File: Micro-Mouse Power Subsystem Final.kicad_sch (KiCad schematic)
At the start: 67 parts, among them J3 USB_C_Receptacle_USB2.0_16P, J4 Battery terminals, J5 Conn_02x16_Odd_Even, Q1 DMP3099L, Q2 2N7002, Q3 DMP3099L, SW1 SW_SPDT, U1 DRV8833PWP, U13 INA219AxD, U2 DRV8833PWP, U3 CH224K, U4 AMS1117-3.3, U5 MT3608, U6 TP4056-42-ESOP8, U7 AMS1117-5.0

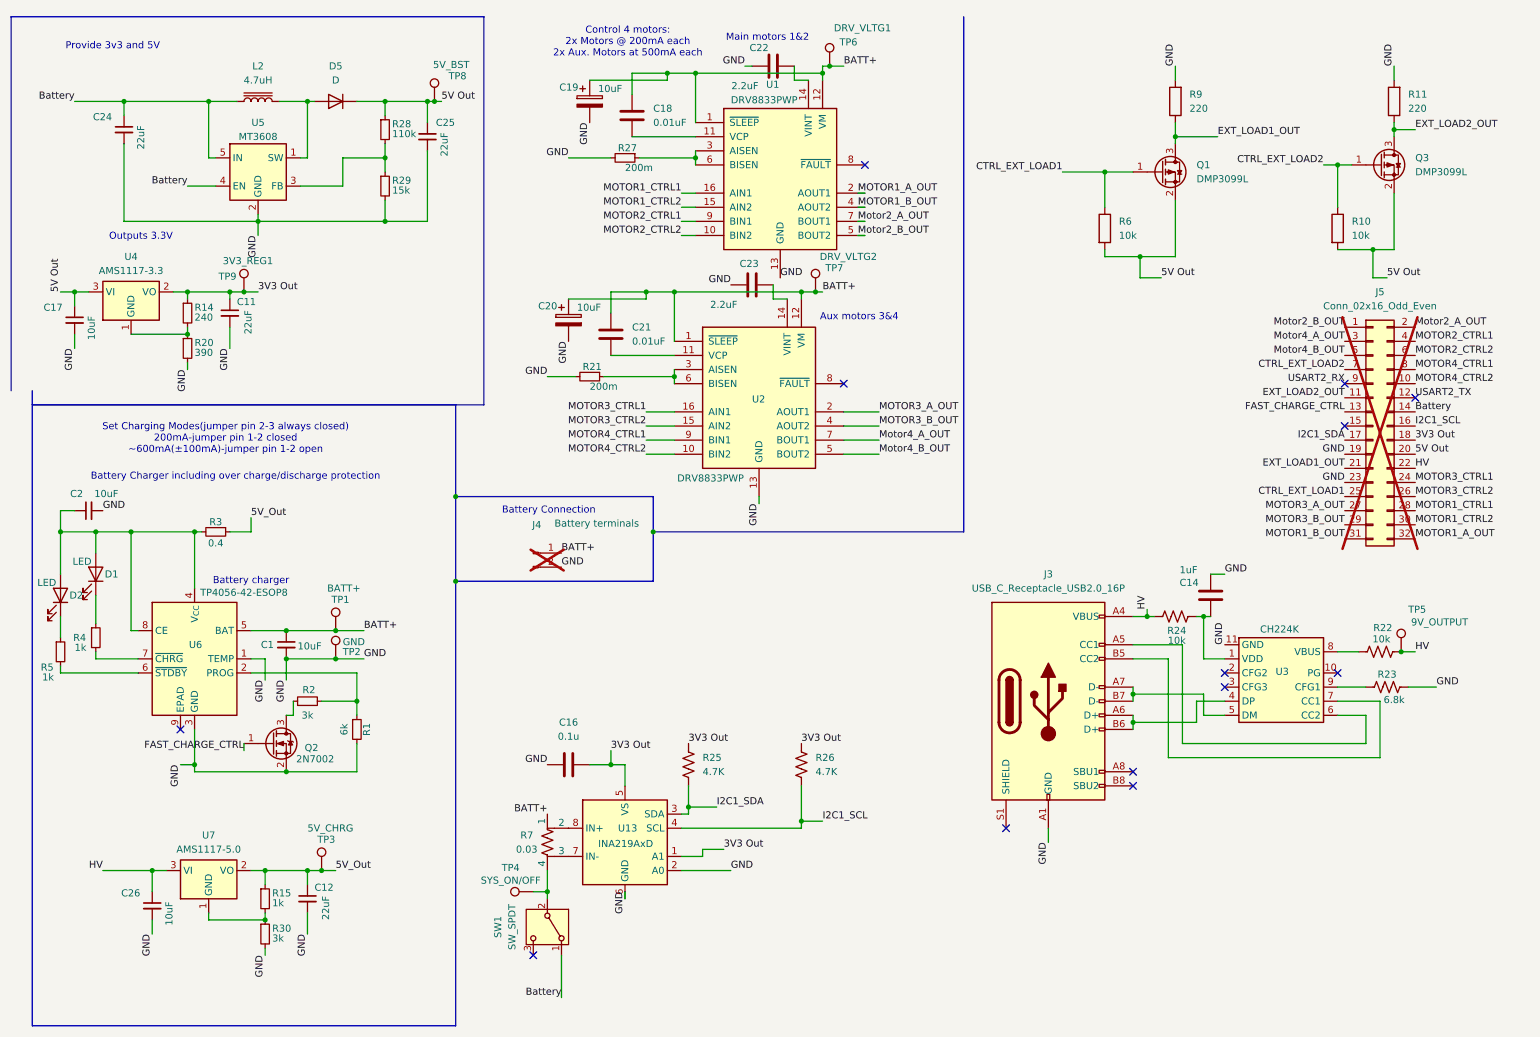
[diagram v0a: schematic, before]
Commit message: Add files via upload
updating the schematic
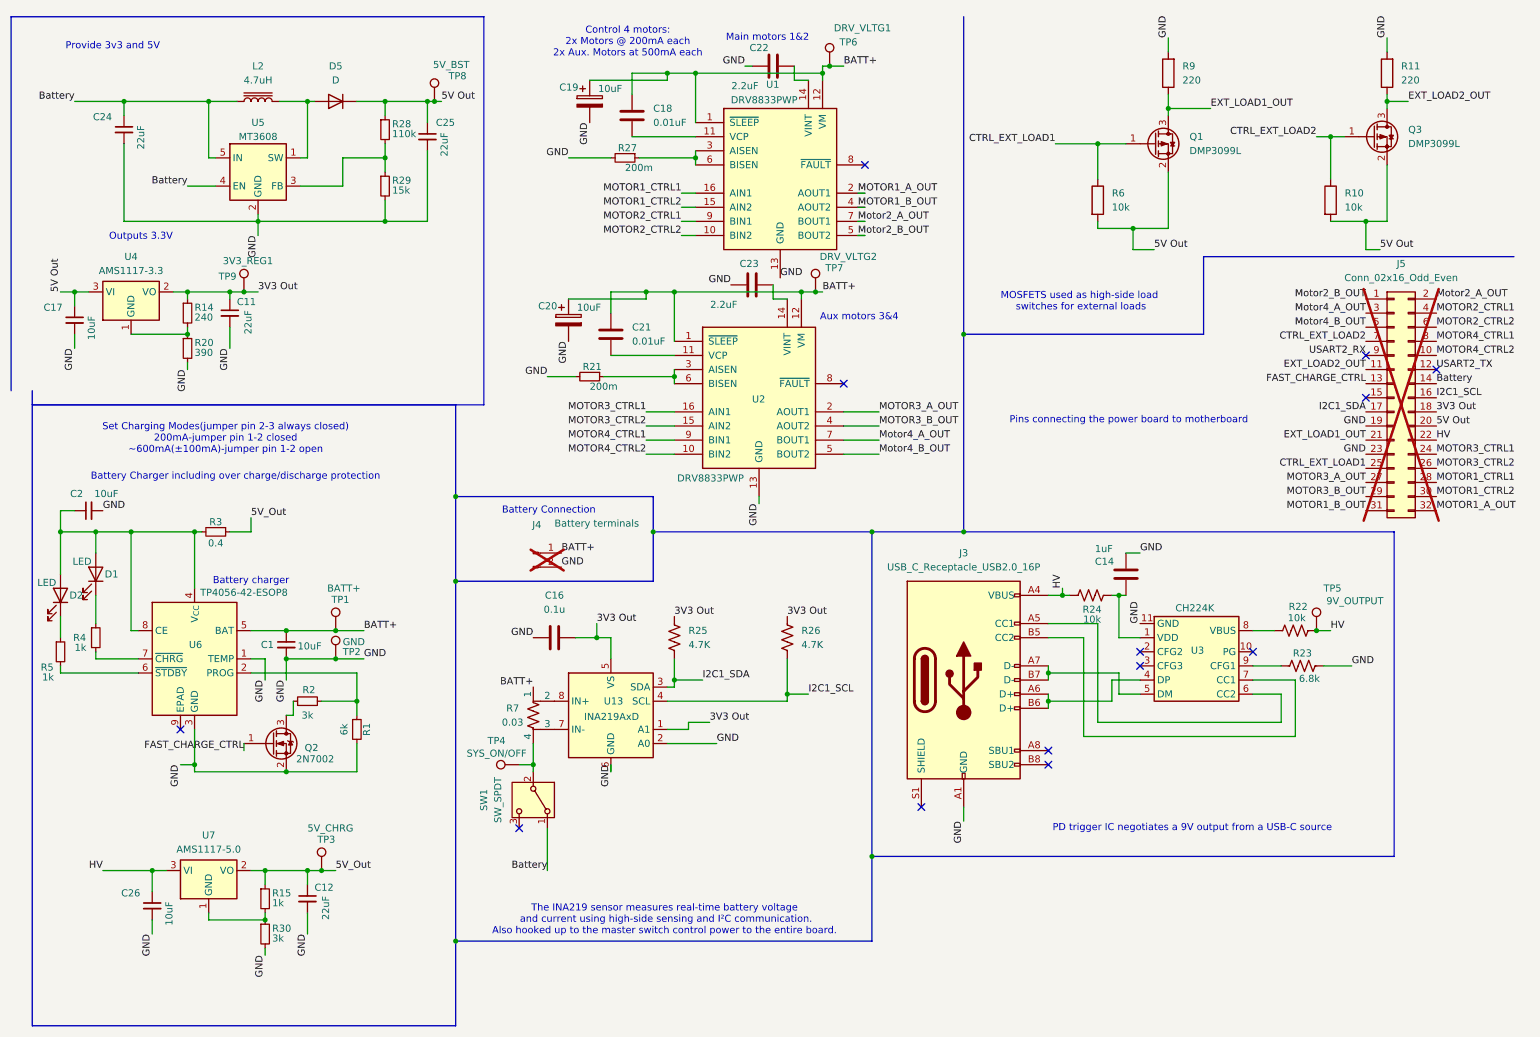
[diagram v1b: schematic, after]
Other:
- note added: "MOSFETS used as high-side load switches for external loads"
- note added: "PD trigger IC negotiates a 9V output from a USB-C source"
- note added: "Pins connecting the power board to motherboard"
- note added: "The INA219 sensor measures real-time battery voltage and current using high-side sensing and I²C communication. Also hooked up to the master switch control power to the entire board."
- moved on the sheet: C14, C16, J3, J5, Q1, Q3, R10, R11, R22, R23, R24, R25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

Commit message: Add files via upload
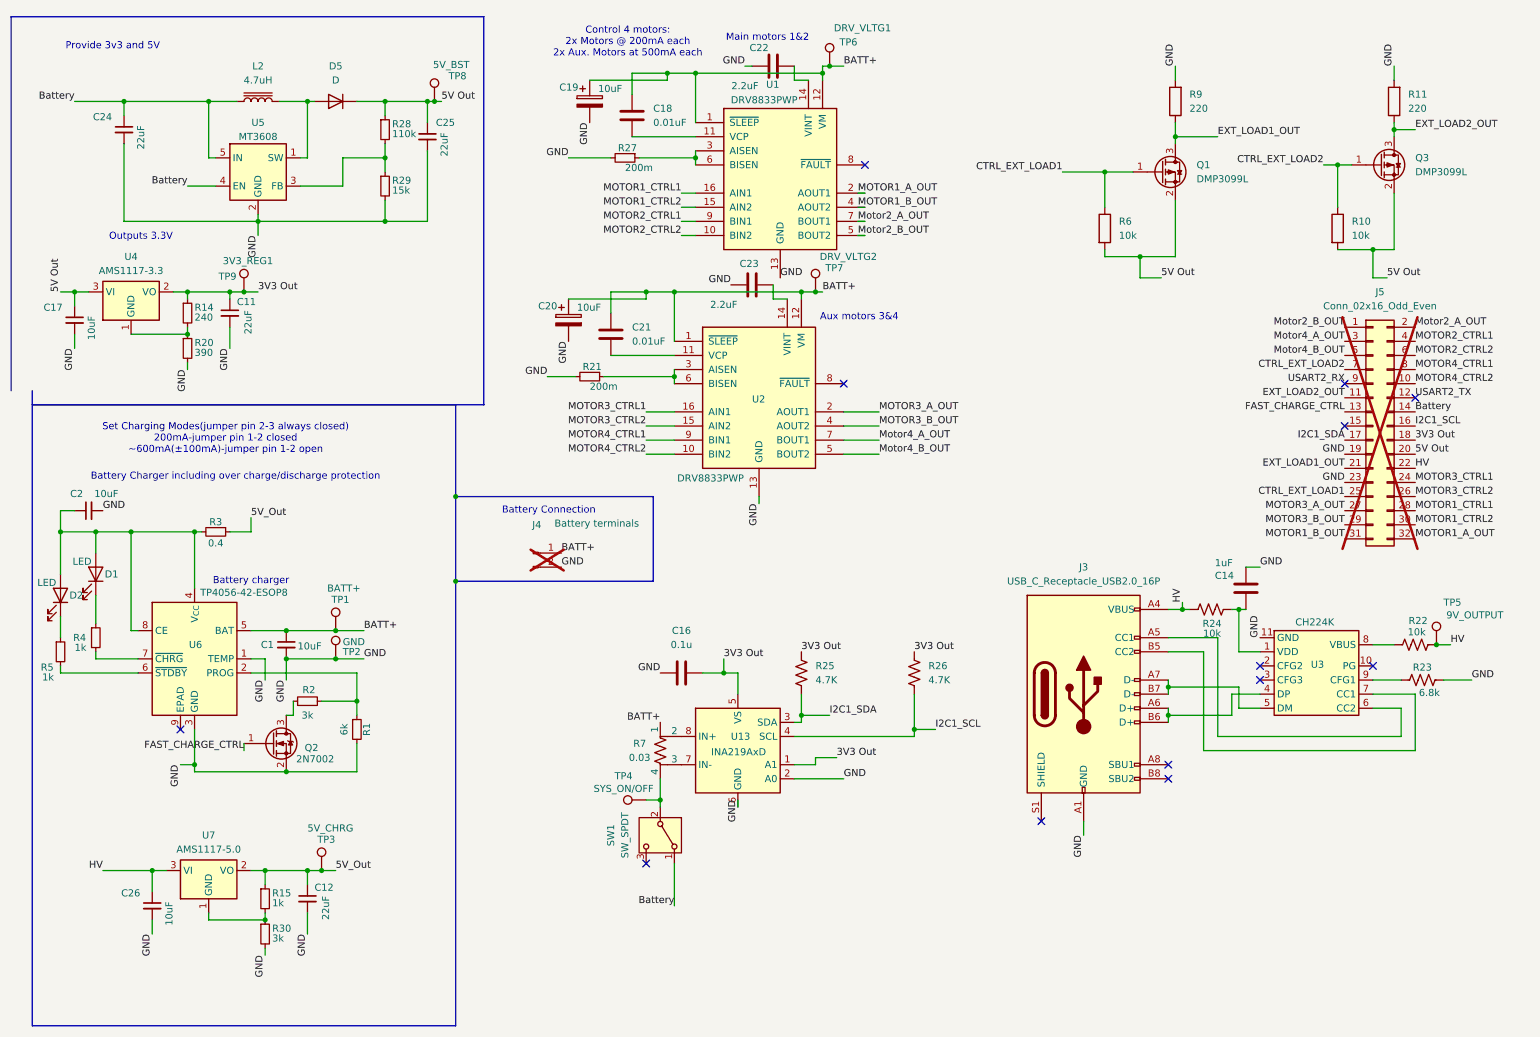
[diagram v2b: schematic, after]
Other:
- note removed: "MOSFETS used as high-side load switches for external loads"
- note removed: "PD trigger IC negotiates a 9V output from a USB-C source"
- note removed: "Pins connecting the power board to motherboard"
- note removed: "The INA219 sensor measures real-time battery voltage and current using high-side sensing and I²C communication. Also hooked up to the master switch control power to the entire board."
- moved on the sheet: C14, C16, J3, J5, Q1, Q3, R10, R11, R22, R23, R24, R25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
